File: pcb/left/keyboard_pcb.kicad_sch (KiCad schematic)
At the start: 42 parts, among them K00 KEYSW, K01 KEYSW, K02 KEYSW, K03 KEYSW, K04 KEYSW, K05 KEYSW, K10 KEYSW, K11 KEYSW, K12 KEYSW, K13 KEYSW, K14 KEYSW, K15 KEYSW, K20 KEYSW, K21 KEYSW, K22 KEYSW, K23 KEYSW, K24 KEYSW, K25 KEYSW, K30 KEYSW, K31 KEYSW, K32 KEYSW, U1 Flippable RP2040 ProMicro/nic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

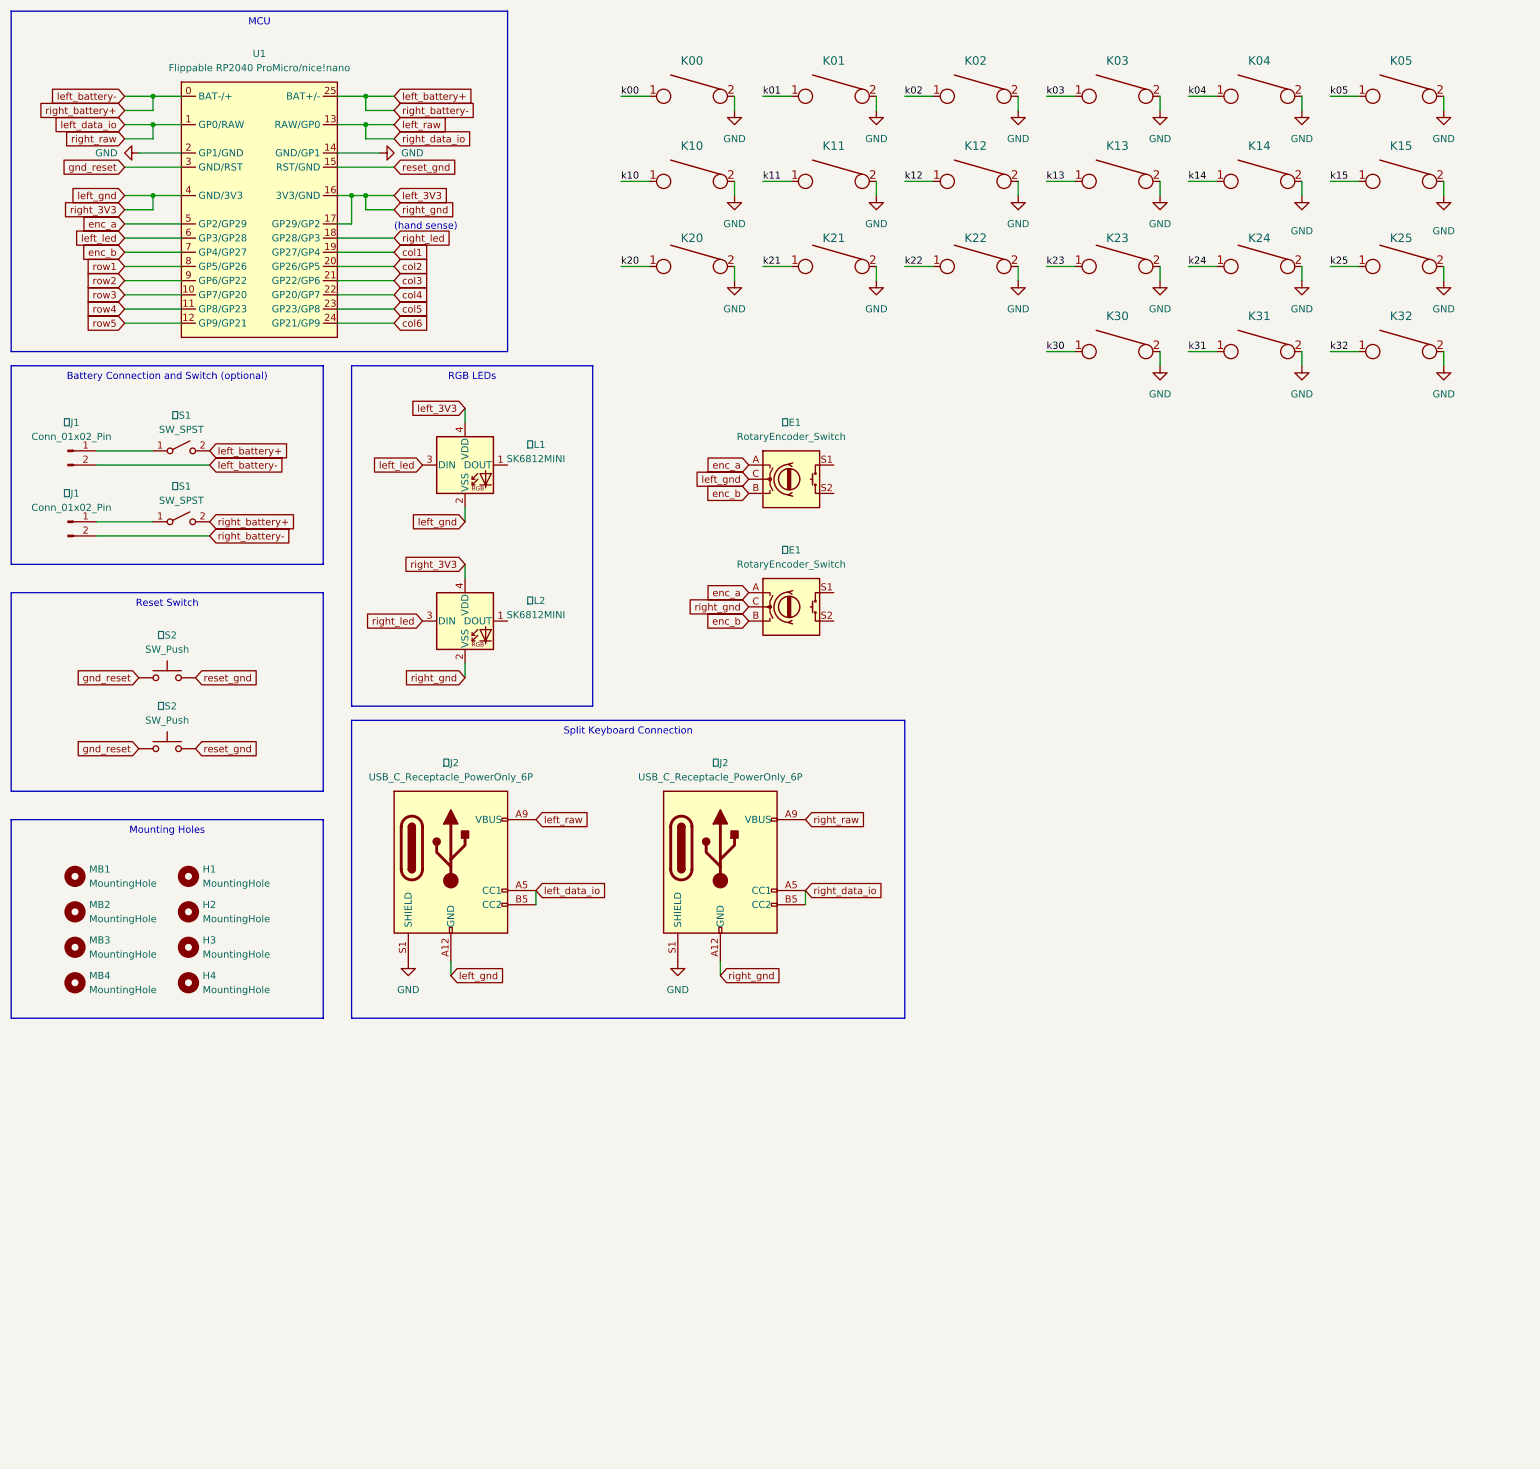
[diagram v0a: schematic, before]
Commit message: Update matrix schematic
 * Add diodes
 * Add 5-way nav. switches
 * Duplicate left to right
 * Tidy layout
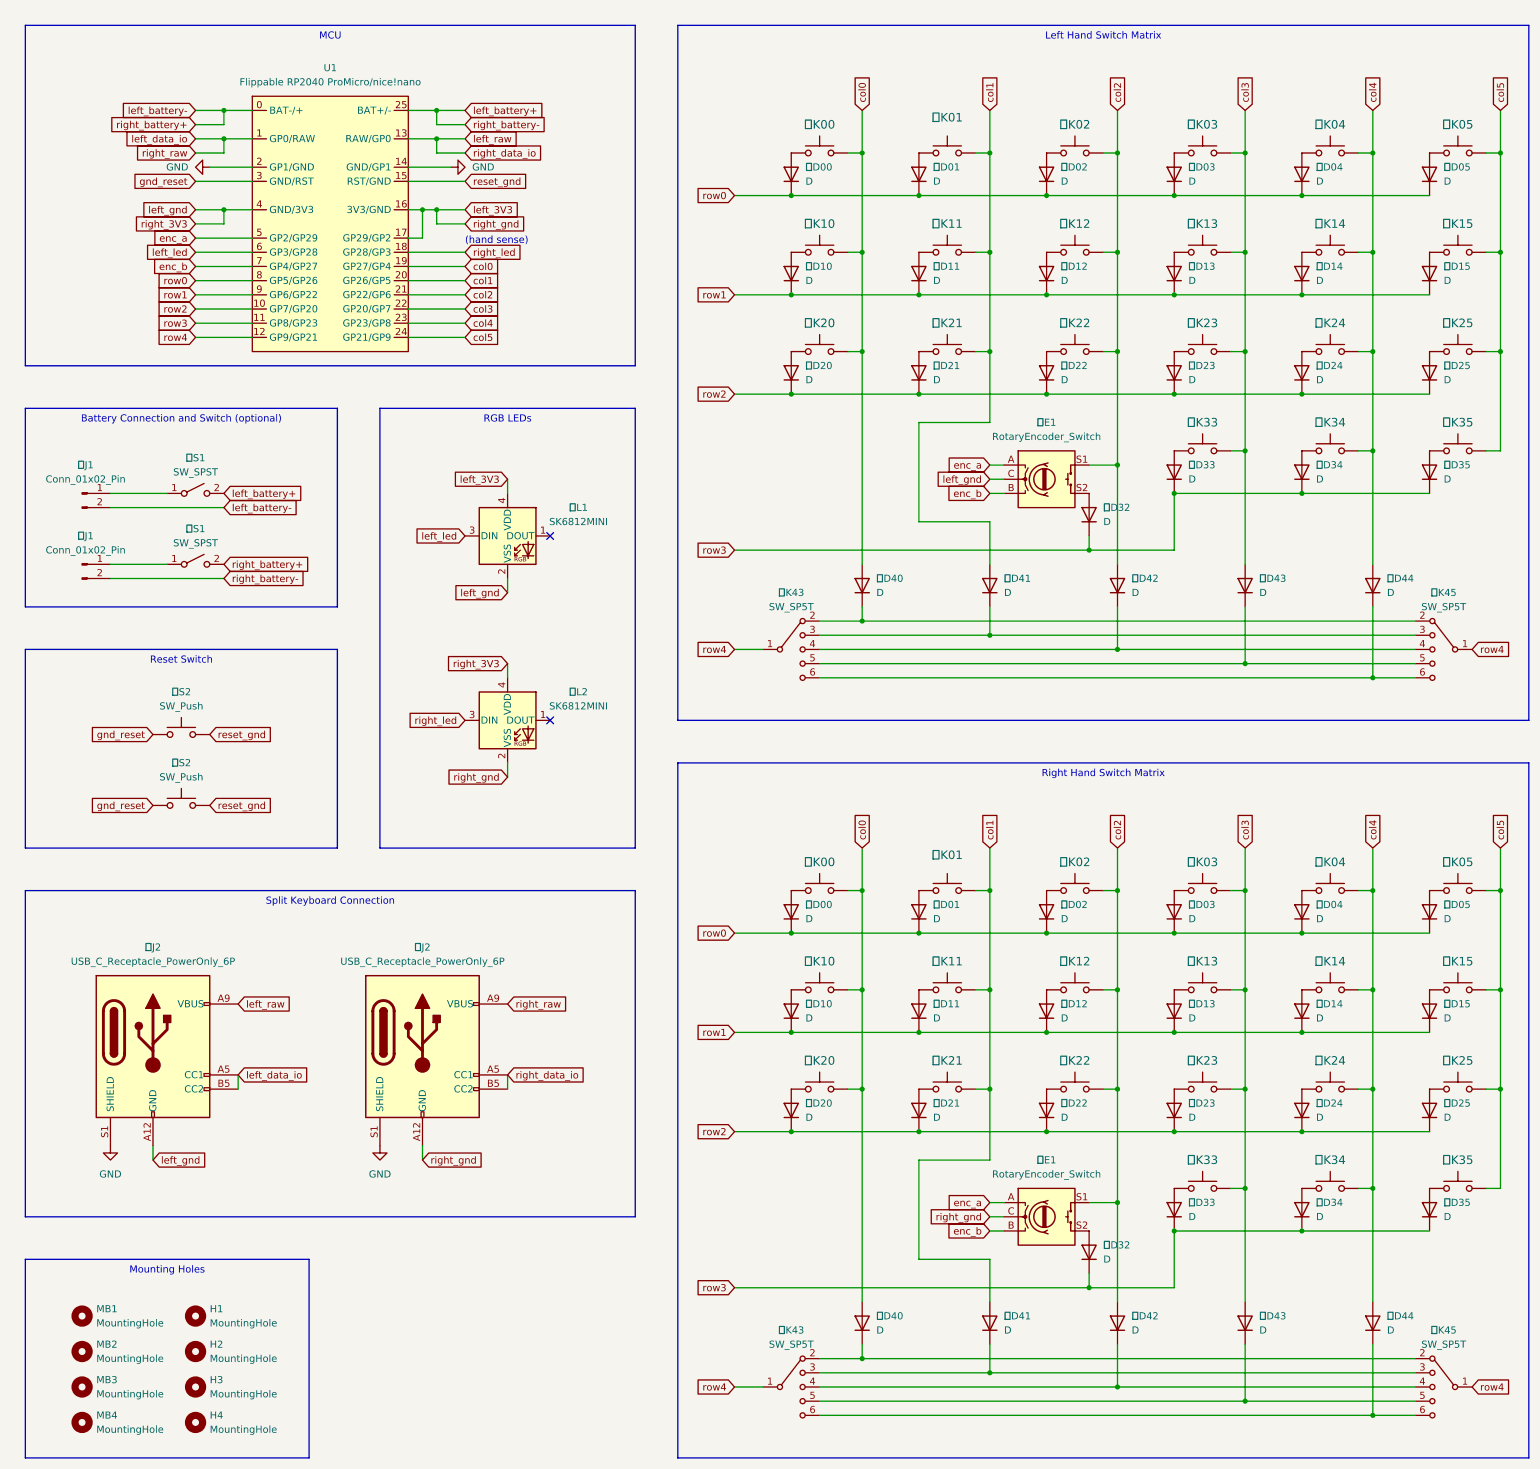
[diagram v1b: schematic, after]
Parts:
- added 右D00, 右D01, 右D02, 右D03, 右D04, 右D05, 右D10, 右D11, 右D12, 右D13, 右D14, 右D15, 右D20, 右D21, 右D22, 右D23, 右D24, 右D25, 右D32, 右D33, 右D34, 右D35, 右D40, 右D41, 右D42, 右D43, 右D44, 左D00, 左D01, 左D02, 左D03, 左D04, 左D05, 左D10, 左D11, 左D12, 左D13, 左D14, 左D15, 左D20, 左D21, 左D22, 左D23, 左D24, 左D25, 左D32, 左D33, 左D34, 左D35, 左D40, 左D41, 左D42, 左D43, 左D44: D, symbol Device:D
- added 右K00, 右K01, 右K02, 右K03, 右K04, 右K05, 右K10, 右K11, 右K12, 右K13, 右K14, 右K15, 右K20, 右K21, 右K22, 右K23, 右K24, 右K25, 右K33, 右K34, 右K35: KEYSW, keyswitches:SW_PG1350_reversible, symbol Switch:SW_Push
- added 右K43, 右K45, 左K43, 左K45: SW_SP5T, symbol _Project Library:SW_SP5T
- 左K00: renamed from K00; symbol keyboard_parts:KEYSW -> Switch:SW_Push
- 左K01: renamed from K01; symbol keyboard_parts:KEYSW -> Switch:SW_Push
- 左K02: renamed from K02; symbol keyboard_parts:KEYSW -> Switch:SW_Push
- 左K03: renamed from K03; symbol keyboard_parts:KEYSW -> Switch:SW_Push
- 左K04: renamed from K04; symbol keyboard_parts:KEYSW -> Switch:SW_Push
- 左K05: renamed from K05; symbol keyboard_parts:KEYSW -> Switch:SW_Push
- 左K10: renamed from K10; symbol keyboard_parts:KEYSW -> Switch:SW_Push
- 左K11: renamed from K11; symbol keyboard_parts:KEYSW -> Switch:SW_Push
- 左K12: renamed from K12; symbol keyboard_parts:KEYSW -> Switch:SW_Push
- 左K13: renamed from K13; symbol keyboard_parts:KEYSW -> Switch:SW_Push
- 左K14: renamed from K14; symbol keyboard_parts:KEYSW -> Switch:SW_Push
- 左K15: renamed from K15; symbol keyboard_parts:KEYSW -> Switch:SW_Push
- 左K20: renamed from K20; symbol keyboard_parts:KEYSW -> Switch:SW_Push
- 左K21: renamed from K21; symbol keyboard_parts:KEYSW -> Switch:SW_Push
- 左K22: renamed from K22; symbol keyboard_parts:KEYSW -> Switch:SW_Push
- 左K23: renamed from K23; symbol keyboard_parts:KEYSW -> Switch:SW_Push
- 左K24: renamed from K24; symbol keyboard_parts:KEYSW -> Switch:SW_Push
- 左K25: renamed from K25; symbol keyboard_parts:KEYSW -> Switch:SW_Push
- 左K33: renamed from K30; symbol keyboard_parts:KEYSW -> Switch:SW_Push
- 左K34: renamed from K31; symbol keyboard_parts:KEYSW -> Switch:SW_Push
- 左K35: renamed from K32; symbol keyboard_parts:KEYSW -> Switch:SW_Push
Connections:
- net col6 is gone; now on net col5: U1.24 (GP21/GP9)
- net k01 is gone; now on net col1: 左K01.1
- net k02 is gone; now on net col2: 左K02.1
- net k03 is gone; now on net col3: 左K03.1
- net k04 is gone; now on net col4: 左K04.1
- net k05 is gone; now on net col5: 左K05.1
- net k10 is gone; now on net col0: 左K10.1
- net k11 is gone; now on net col1: 左K11.1
- net k12 is gone; now on net col2: 左K12.1
- net k13 is gone; now on net col3: 左K13.1
- net k14 is gone; now on net col4: 左K14.1
- net k15 is gone; now on net col5: 左K15.1
- net k20 is gone; now on net col0: 左K20.1
- net k21 is gone; now on net col1: 左K21.1
- net k22 is gone; now on net col2: 左K22.1
- net k23 is gone; now on net col3: 左K23.1
- net k24 is gone; now on net col4: 左K24.1
- net k25 is gone; now on net col5: 左K25.1
- net k30 is gone; now on net col3: 左K33.1
- net k31 is gone; now on net col4: 左K34.1
- net k32 is gone; now on net col5: 左K35.1
- net row5 is gone; now on net row4: U1.12 (GP9/GP21)
- net GND: no longer 左K00.2, 左K01.2, 左K02.2, 左K03.2, 左K04.2, 左K05.2, 左K10.2, 左K11.2, 左K12.2, 左K13.2, 左K14.2, 左K15.2, 左K20.2, 左K21.2, 左K22.2, 左K23.2, 左K24.2, 左K25.2, 左K33.2, 左K34.2, 左K35.2
- net col1: now also U1.20 (GP26/GP5), 右D41.2 (A), 右K01.1, 右K11.1, 右K21.1, 左D41.2 (A); no longer U1.19 (GP27/GP4)
- net col2: now also U1.21 (GP22/GP6), 右E1.S1, 左E1.S1, 右D42.2 (A), 右K02.1, 右K12.1, 右K22.1, 左D42.2 (A); no longer U1.20 (GP26/GP5)
- net col3: now also U1.22 (GP20/GP7), 右D43.2 (A), 右K03.1, 右K13.1, 右K23.1, 右K33.1, 左D43.2 (A); no longer U1.21 (GP22/GP6)
- net col4: now also U1.23 (GP23/GP8), 右D44.2 (A), 右K04.1, 右K14.1, 右K24.1, 右K34.1, 左D44.2 (A); no longer U1.22 (GP20/GP7)
- net col5: now also 右K05.1, 右K15.1, 右K25.1, 右K35.1; no longer U1.23 (GP23/GP8)
- net row1: now also U1.9 (GP6/GP22), 右D10.1 (K), 右D11.1 (K), 右D12.1 (K), 右D13.1 (K), 右D14.1 (K), 右D15.1 (K), 左D10.1 (K), 左D11.1 (K), 左D12.1 (K), 左D13.1 (K), 左D14.1 (K), 左D15.1 (K); no longer U1.8 (GP5/GP26)
- net row2: now also U1.10 (GP7/GP20), 右D20.1 (K), 右D21.1 (K), 右D22.1 (K), 右D23.1 (K), 右D24.1 (K), 右D25.1 (K), 左D20.1 (K), 左D21.1 (K), 左D22.1 (K), 左D23.1 (K), 左D24.1 (K), 左D25.1 (K); no longer U1.9 (GP6/GP22)
- net row3: now also U1.11 (GP8/GP23), 右D32.1 (K), 右D33.1 (K), 右D34.1 (K), 右D35.1 (K), 左D32.1 (K), 左D33.1 (K), 左D34.1 (K), 左D35.1 (K); no longer U1.10 (GP7/GP20)
- net row4: now also 右K43.1, 右K45.1, 左K43.1, 左K45.1; no longer U1.11 (GP8/GP23)
- net at 右E1.S2: now also 右D32.2 (A)
- net at 左E1.S2: now also 左D32.2 (A)
- net k00 renamed col0
- net col0: now also U1.19 (GP27/GP4), 右D40.2 (A), 右K00.1, 右K10.1, 右K20.1, 左D40.2 (A)
- new net: 右D21.2 (A), 右K21.2
- new net: 左D35.2 (A), 左K35.2
- new net: 左D13.2 (A), 左K13.2
- new net: 右D22.2 (A), 右K22.2
- new net: 左D24.2 (A), 左K24.2
- new net: 右D00.2 (A), 右K00.2
- new net: 右D23.2 (A), 右K23.2
- new net: 左D05.2 (A), 左K05.2
- new net: 右D25.2 (A), 右K25.2
- new net: 右D01.2 (A), 右K01.2
- new net: 右D02.2 (A), 右K02.2
- new net: 左D20.2 (A), 左K20.2
- new net: 左D11.2 (A), 左K11.2
- new net: 右D34.2 (A), 右K34.2
- new net: 右D24.2 (A), 右K24.2
- new net: 右D35.2 (A), 右K35.2
- new net: 左D00.2 (A), 左K00.2
- new net: 右D20.2 (A), 右K20.2
- new net: 右D14.2 (A), 右K14.2
- new net: 左D14.2 (A), 左K14.2
- new net: 左D15.2 (A), 左K15.2
- new net: 左D42.1 (K), 左K43.4, 左K45.4
- new net: 右D03.2 (A), 右K03.2
- new net: 右D33.2 (A), 右K33.2
- new net: 右D04.2 (A), 右K04.2
- new net: 右D41.1 (K), 右K43.3, 右K45.3
- new net: 右D05.2 (A), 右K05.2
- new net: 左D03.2 (A), 左K03.2
- new net: 右D44.1 (K), 右K43.6, 右K45.6
- new net: 左D43.1 (K), 左K43.5, 左K45.5
- new net: 左D22.2 (A), 左K22.2
- new net: 左D40.1 (K), 左K43.2, 左K45.2
- new net: 左D41.1 (K), 左K43.3, 左K45.3
- new net: 左D44.1 (K), 左K43.6, 左K45.6
- new net: 左D02.2 (A), 左K02.2
- new net: 右D13.2 (A), 右K13.2
- new net: 左D33.2 (A), 左K33.2
- new net: 右D43.1 (K), 右K43.5, 右K45.5
- new net: 右D42.1 (K), 右K43.4, 右K45.4
- new net: 右D11.2 (A), 右K11.2
- new net: 左D04.2 (A), 左K04.2
- new net: 左D12.2 (A), 左K12.2
- new net: 左D23.2 (A), 左K23.2
- new net: 右D10.2 (A), 右K10.2
- new net: 左D25.2 (A), 左K25.2
- new net: 右D12.2 (A), 右K12.2
- new net: 左D10.2 (A), 左K10.2
- new net: 左D01.2 (A), 左K01.2
- new net: 左D34.2 (A), 左K34.2
- new net: 右D40.1 (K), 右K43.2, 右K45.2
- new net: 左D21.2 (A), 左K21.2
- new net: 右D15.2 (A), 右K15.2
- new net row0: U1.8 (GP5/GP26), 右D00.1 (K), 右D01.1 (K), 右D02.1 (K), 右D03.1 (K), 右D04.1 (K), 右D05.1 (K), 左D00.1 (K), 左D01.1 (K), 左D02.1 (K), 左D03.1 (K), 左D04.1 (K), 左D05.1 (K)
- no-connect marks 0 -> 2
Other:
- moved on the sheet: H1, H2, H3, H4, MB1, MB2, MB3, MB4, U1, 右J1, 右J2, 右L2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
